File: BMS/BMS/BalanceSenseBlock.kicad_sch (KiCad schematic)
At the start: 7 parts

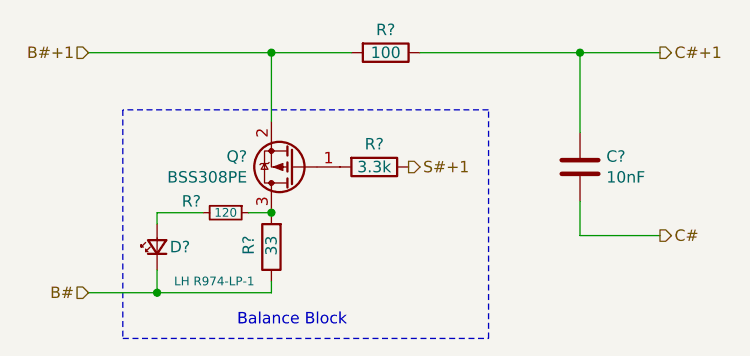
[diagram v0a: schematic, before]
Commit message: BMS
updated BMS schematic with new global tags
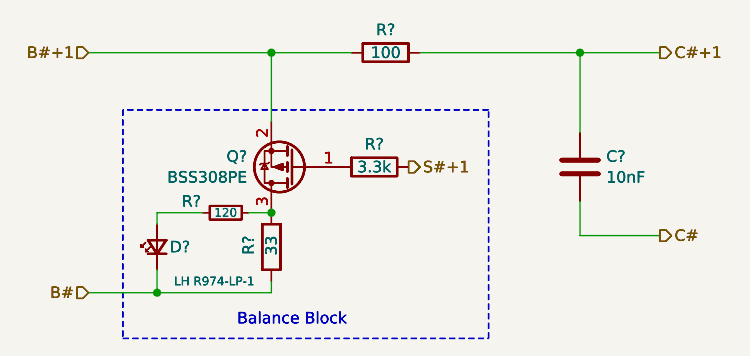
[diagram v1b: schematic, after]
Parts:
- added C?: 10nF, Capacitor_SMD:C_0805_2012Metric_Pad1.18x1.45mm_HandSolder, symbol Device:C
- added D?: LH R974-LP-1, LED_SMD:LED_0805_2012Metric_Pad1.15x1.40mm_HandSolder, symbol Device:LED_Small
- added Q?: BSS308PE, Package_TO_SOT_SMD:SOT-23, symbol Transistor_FET:BSS84
- added R?: 120, Resistor_SMD:R_0805_2012Metric_Pad1.20x1.40mm_HandSolder, symbol Device:R_Small
- added R?: 100, Resistor_SMD:R_0805_2012Metric_Pad1.20x1.40mm_HandSolder, symbol Device:R
- added R?: 33, Resistor_SMD:R_2512_6332Metric_Pad1.40x3.35mm_HandSolder, symbol Device:R
- added R?: 3.3k, Resistor_SMD:R_0805_2012Metric_Pad1.20x1.40mm_HandSolder, symbol Device:R
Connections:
- net B#: now also D?.1 (K), R?.1
- net B#+1: now also Q?.2 (S), R?.2
- net C#: now also C?.2
- net C#+1: now also C?.1, R?.1
- net S#+1: now also R?.1
- net at Q?.1 (G), R?.2: now also Q?.1 (G), R?.2
- net at Q?.3 (D), R?.1, R?.2: now also Q?.3 (D), R?.1, R?.2
- net at D?.2 (A), R?.2: now also D?.2 (A), R?.2
